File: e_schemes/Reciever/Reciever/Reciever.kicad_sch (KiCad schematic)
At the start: 31 parts, among them J1 Conn_01x03, J2 Conn_01x03, Q1 AO3400A, SW1 SW_Push, SW2 SW_Push, SW3 SW_Reload, U1 ESP32-WROOM-32E

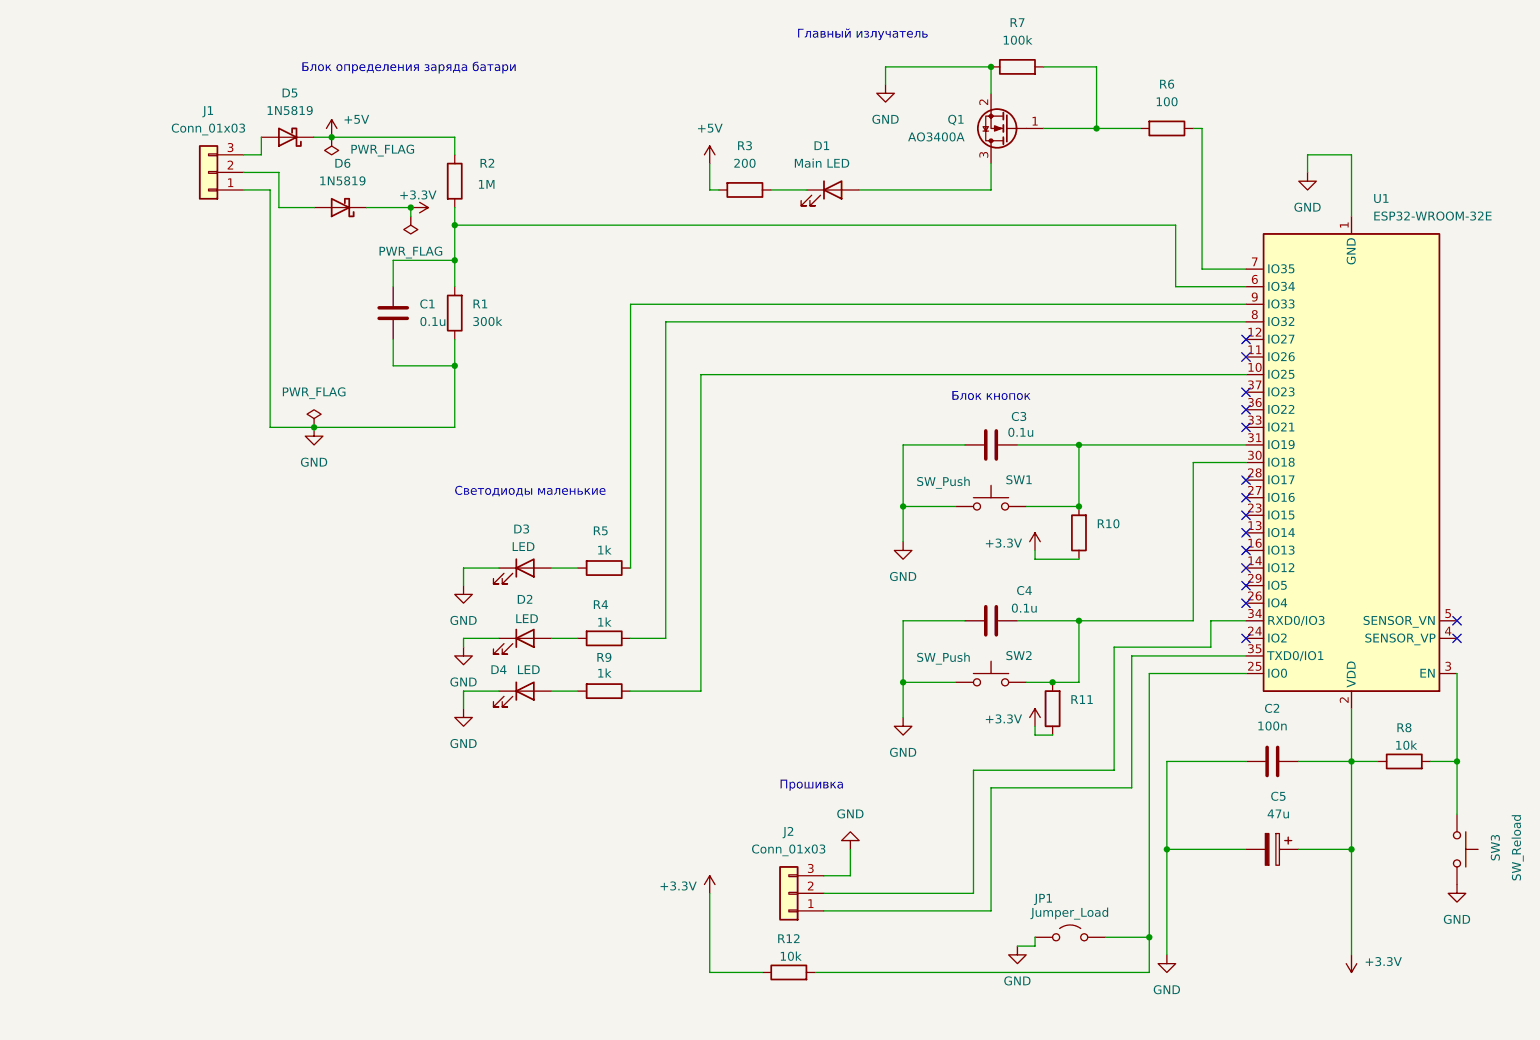
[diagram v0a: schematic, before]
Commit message: ADD: Добавлены  электросхемы
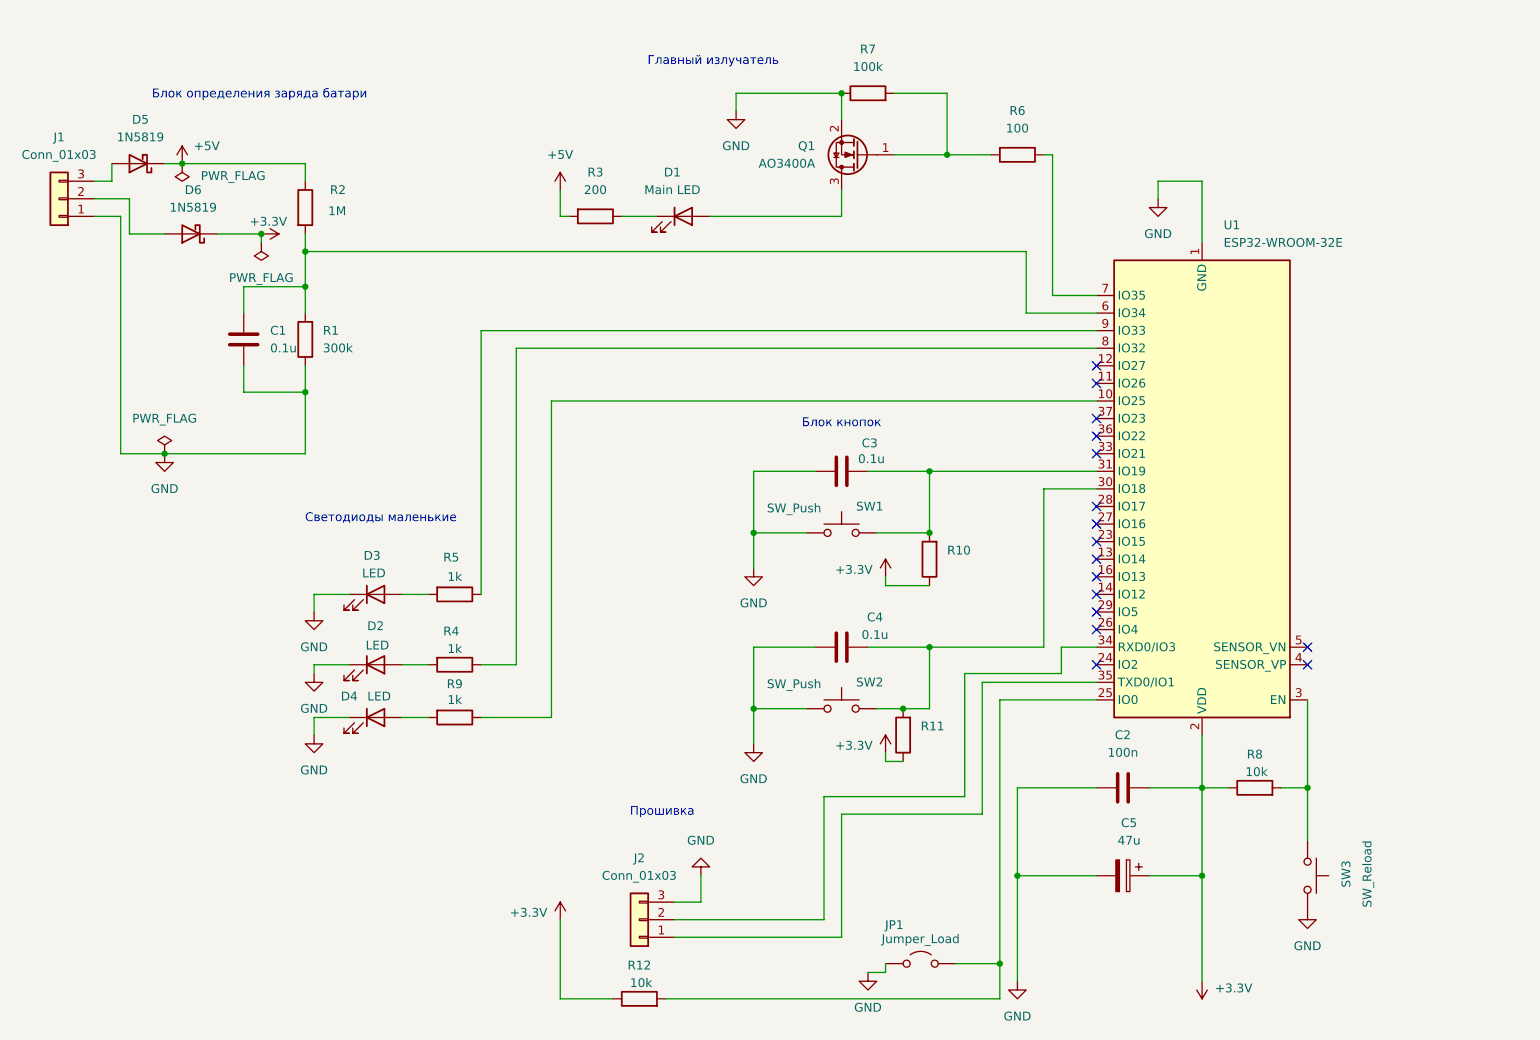
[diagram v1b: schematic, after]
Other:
- company: SF-DEV -> (none)
- title: Схема передатчика -> (none)
- moved on the sheet: C1, C2, C3, C4, C5, D1, D2, D3, D4, D5, D6, J1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
